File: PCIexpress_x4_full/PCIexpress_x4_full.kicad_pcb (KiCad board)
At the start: 4 copper layers, 312 x 111.2 mm, 18 parts, among them J1 PCIexpress_bracket, J2 PCIexpress_x4

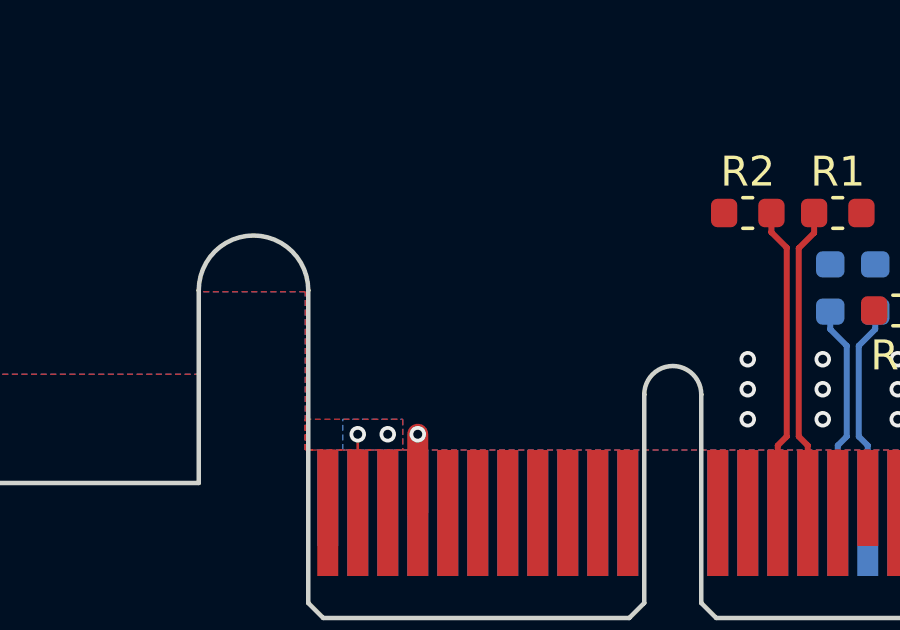
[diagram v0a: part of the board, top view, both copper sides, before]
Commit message: KiCad 6 update
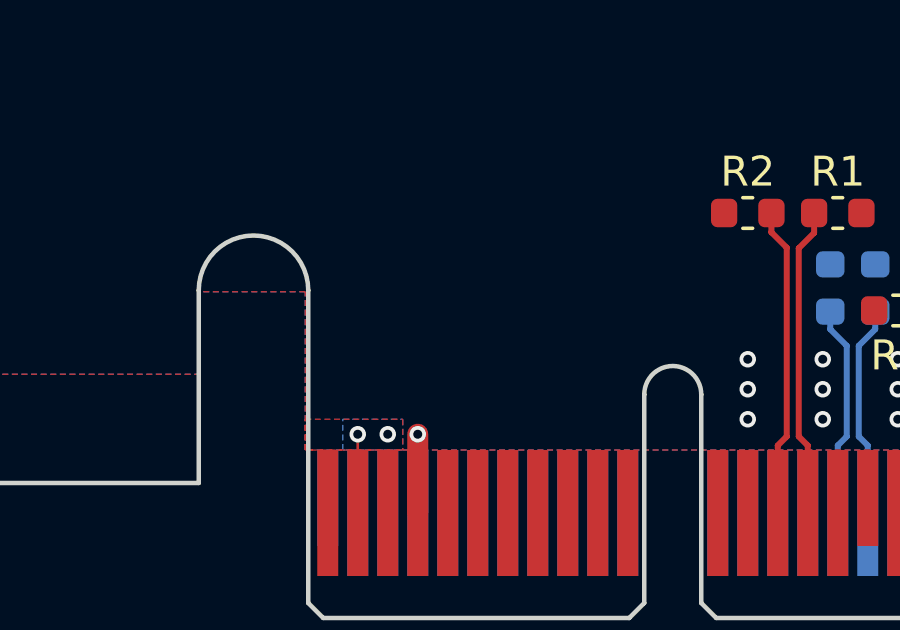
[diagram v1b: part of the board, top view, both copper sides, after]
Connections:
- net /~PERST renamed /~{PERST}
- net /~PRSNT1 renamed /~{PRSNT1}
- net /~PRSNT2x1 renamed /~{PRSNT2x1}
- net /~PRSNT2x4 renamed /~{PRSNT2x4}
- net /~TRST renamed /~{TRST}
- net /~WAKE renamed /~{WAKE}
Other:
- net class Default removed
- net class Diff-100-PCIe removed
- net class JLC2313-100d-3.5 removed
- net class JLC2313-100d-4 removed
- net class JLC7628-100d-8 removed
